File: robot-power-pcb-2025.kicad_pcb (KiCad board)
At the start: 2 copper layers, 100 x 200 mm, 39 parts, among them J1 B14B-PHDSS, J10 B2B-PH, J11 B2B-PH, J12 B4B-PH, J13 B4B-PH, J14 XT60, J2 XT60, J3 B2B-PH, J4 B2B-PH, J5 XT30, J6 XT30, J7 B2B-PH, J8 B2B-PH, J9 B2B-PH, Q1 IRLZ44N, U1 BigTreeTechV1.3_Module, U2 BigTreeTechV1.3_Module, U3 SBR-L, U4 SBR-R

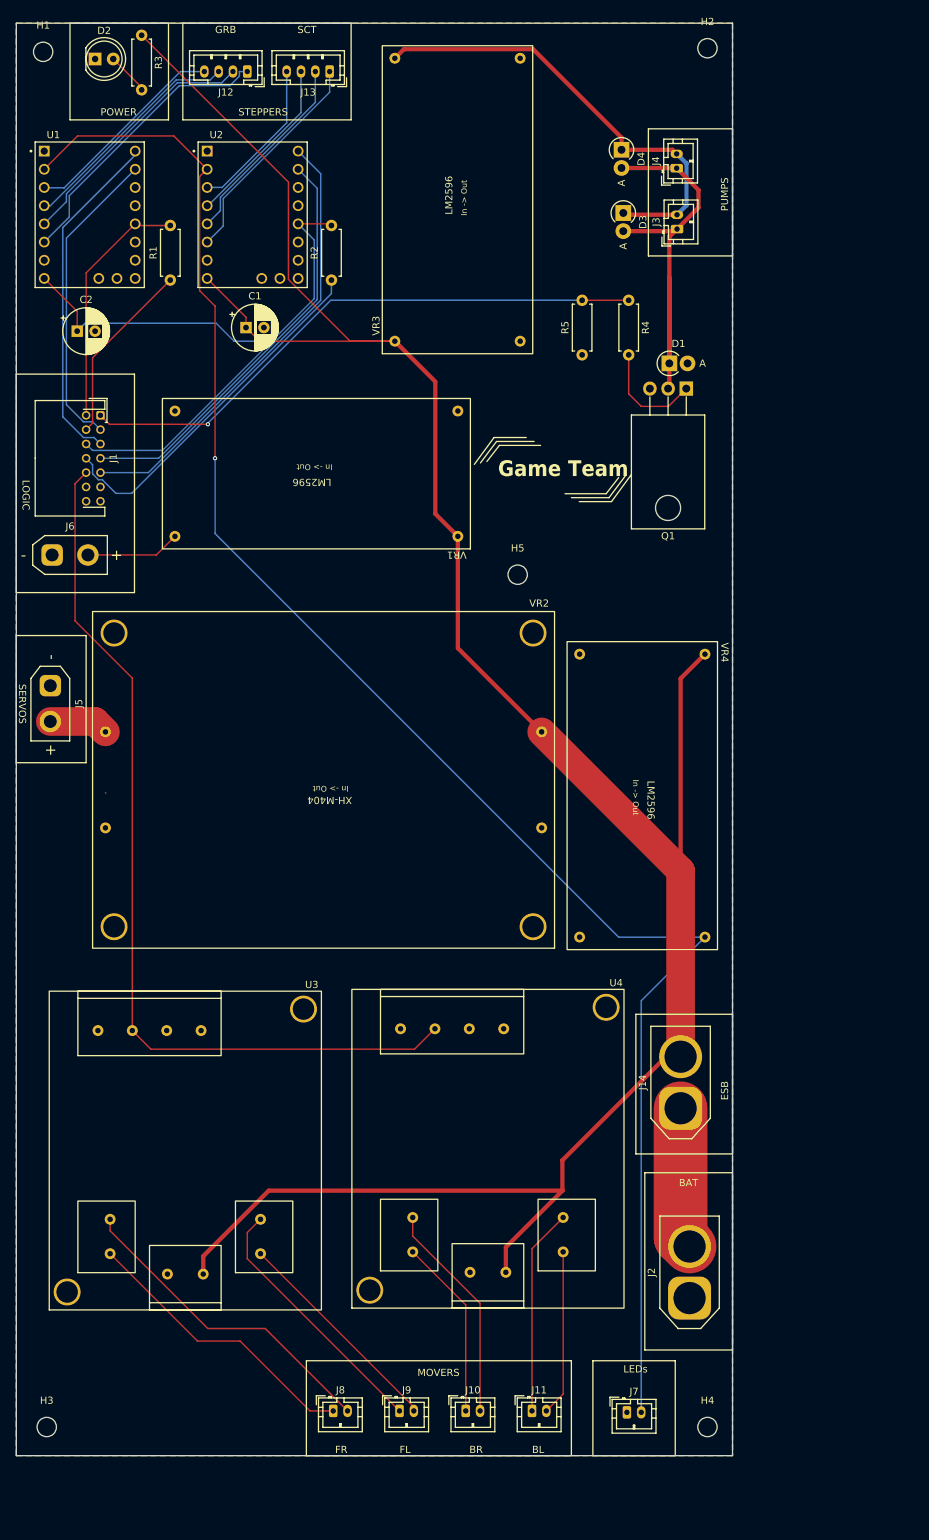
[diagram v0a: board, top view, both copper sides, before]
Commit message: First commit
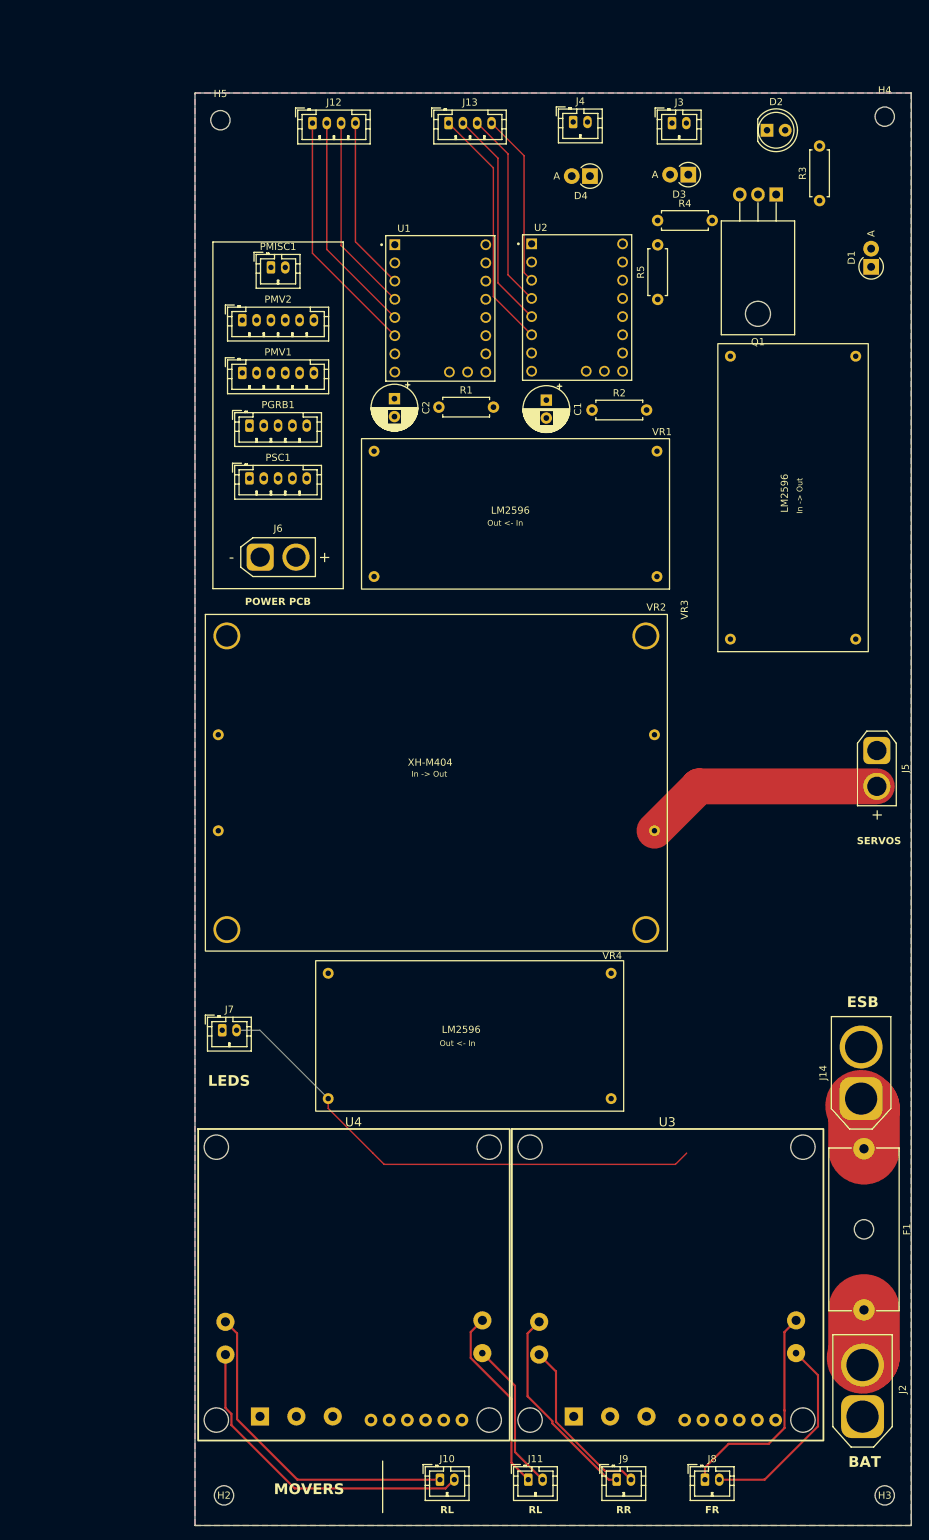
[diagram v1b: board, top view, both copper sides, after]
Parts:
- removed H1: MountingHole, MountingHole:MountingHole_2.7mm_M2.5
- removed J1: B14B-PHDSS, Connector_JST:JST_PHD_S14B-PHDSS_2x07_P2.00mm_Horizontal
- added F1: Fuse, Fuse:Fuseholder_Cylinder-5x20mm_Schurter_0031_8201_Horizontal_Open, F.Cu at (264.6, 195.4)
- added PGRB1: PH5A, Connector_JST:JST_PH_B5B-PH-K_1x05_P2.00mm_Vertical, F.Cu at (178.8, 94.4)
- added PMISC1: PH2A, Connector_JST:JST_PH_B2B-PH-K_1x02_P2.00mm_Vertical, F.Cu at (181.8, 72.3)
- added PMV1: PH6A, Connector_JST:JST_PH_B6B-PH-K_1x06_P2.00mm_Vertical, F.Cu at (177.8, 87.1)
- added PMV2: PH6A, Connector_JST:JST_PH_B6B-PH-K_1x06_P2.00mm_Vertical, F.Cu at (177.8, 79.7)
- added PSC1: PH5A, Connector_JST:JST_PH_B5B-PH-K_1x05_P2.00mm_Vertical, F.Cu at (178.8, 101.8)
- D2: value LED -> LED_Green
- J5, J6: footprint Connector_AMASS:AMASS_XT30UPB-M_1x02_P5.0mm_Vertical -> Connector_AMASS:AMASS_XT30U-M_1x02_P5.0mm_Vertical
- R1, R2: value 10k -> 1k
- R3: value 1.1k -> 430
- U3: value SBR-L -> L298N_Bridge; footprint Project:Sabertooth_2X5 -> Project:L298N_Bridge
- U4: value SBR-R -> L298N_Bridge; footprint Project:Sabertooth_2X5 -> Project:L298N_Bridge
- moved H2 213.0 mm to (175.2, 243.8)
- moved H4 184.6 mm to (267.5, 51.3)
- moved H3 117.4 mm to (267.5, 243.8)
- moved J5 115.8 mm to (266.4, 139.8)
- moved R3 97.4 mm to (258.4, 63.0), turned to 90 degrees
- moved D2 94.3 mm to (251.1, 53.2)
- moved J7 77.7 mm to (175.0, 178.8)
- moved H5 75.8 mm to (174.8, 51.8)
- moved VR2 67.4 mm to (172.7, 120.8), turned to 0 degrees
- moved U3 67.1 mm to (215.4, 236.1), turned to 0 degrees
- moved VR4 66.8 mm to (231.1, 190.2), turned to 180 degrees
- moved VR3 62.7 mm to (244.2, 126.0)
- moved J8 52.8 mm to (242.4, 241.6)
- moved U1 50.7 mm to (205.4, 78.1)
- moved U2 47.1 mm to (224.6, 78.0)
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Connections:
- net /grb-tx renamed GRB_TX
- net /pump-rly renamed PUMP_RLY
- net /sc-tx renamed SC_TX
- J2 pad 2: Net-(J14-Pin_1) -> Net-(J2-Pin_2)
- R1 pad 1: /grb-rx -> GRB_RX
- R2 pad 1: /sc-rx -> SC_RX
- U1 pad 1: GND -> GRB_EN
- U1 pad 7: /grb-step -> GRB_STEP
- U1 pad 8: /grb-dir -> GRB_DIR
- U2 pad 1: GND -> SC_EN
- U2 pad 7: /sc-step -> SC_STEP
- U2 pad 8: /sc-dir -> SC_DIR
- U3 pad 1: GND -> +16.8V
- U3 pad 10: Net-(J8-Pin_2) -> Net-(J9-Pin_1)
- U3 pad 2: +16.8V -> GND
- U3 pad 3: GND -> +5V
- U3 pad 4: unconnected-(U3-5V-Pad4) -> L298N_L_ENA
- U3 pad 5: /sbr -> L298N_L_IN1
- U3 pad 6: unconnected-(U3-S2-Pad6) -> L298N_L_IN2
- U3 pad 7: Net-(J9-Pin_1) -> L298N_L_IN3
- U3 pad 8: Net-(J9-Pin_2) -> L298N_L_IN4
- U3 pad 9: Net-(J8-Pin_1) -> L298N_L_ENB
- U4 pad 1: GND -> +16.8V
- U4 pad 10: Net-(J10-Pin_2) -> Net-(J10-Pin_1)
- U4 pad 2: +16.8V -> GND
- U4 pad 3: GND -> +5V
- U4 pad 4: unconnected-(U4-5V-Pad4) -> L298N_R_ENA
- U4 pad 5: /sbr -> L298N_R_IN1
- U4 pad 6: unconnected-(U4-S2-Pad6) -> L298N_R_IN2
- U4 pad 7: Net-(J11-Pin_1) -> L298N_R_IN3
- U4 pad 8: Net-(J11-Pin_2) -> L298N_R_IN4
- U4 pad 9: Net-(J10-Pin_1) -> L298N_R_ENB
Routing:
- net +16.8V: track 402.0 -> 0.00 mm, vias 1 -> 0
- net +5V: track 240.9 -> 72.1 mm, vias 1 -> 0
- net /sbr: track 126.4 -> 0.00 mm
- net PUMP_RLY: track 81.5 -> 0.00 mm, vias 1 -> 0
- net +12V: track 64.2 -> 0.00 mm
- net /sc-dir: track 62.8 -> 0.00 mm
- net Net-(D1-K): track 61.2 -> 0.00 mm
- net /sc-step: track 58.7 -> 0.00 mm
- net SC_TX: track 57.1 -> 0.00 mm
- net /sc-rx: track 50.5 -> 0.00 mm
- net /grb-dir: track 48.1 -> 0.00 mm
- net /grb-step: track 43.0 -> 0.00 mm
- net GRB_TX: track 34.6 -> 0.00 mm
- net /grb-rx: track 25.7 -> 0.00 mm
- net +5VPWR: track 8.30 -> 33.6 mm
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- added copper zone on B.Cu, net +16.8V
- removed copper zone on B.Cu, net GND
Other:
- board text added: "LEDS"
- board text added: "RL"
- board text added: "RR"
- board text removed: "BL"
- board text removed: "BR"
- board text removed: "FL"
- board text removed: "GRB"
- board text removed: "Game Team"
- board text removed: "INPUT : 15-17V 20A"
- board text removed: "LEDs"
- board text removed: "LOGIC"
- board text removed: "NOTICE"
- board text removed: "POWER"
- board text removed: "PUMPS"
- board text removed: "SCT"
- board text removed: "STEPPERS"
